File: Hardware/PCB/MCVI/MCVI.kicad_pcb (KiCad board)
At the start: 2 copper layers, 125.5 x 138 mm, 69 parts, among them IC1 TL074, IC2 TL074, J1 Synth_power_2x5, J10 AudioJack2, J11 AudioJack2, J12 AudioJack2, J13 AudioJack2, J14 AudioJack2, J15 AudioJack2, J16 AudioJack2, J2 10 pin header, J3 3 pin Molex header, J4 2 pin Molex header, J8 10 pin socket, J9 AudioJack2, U1 6N137

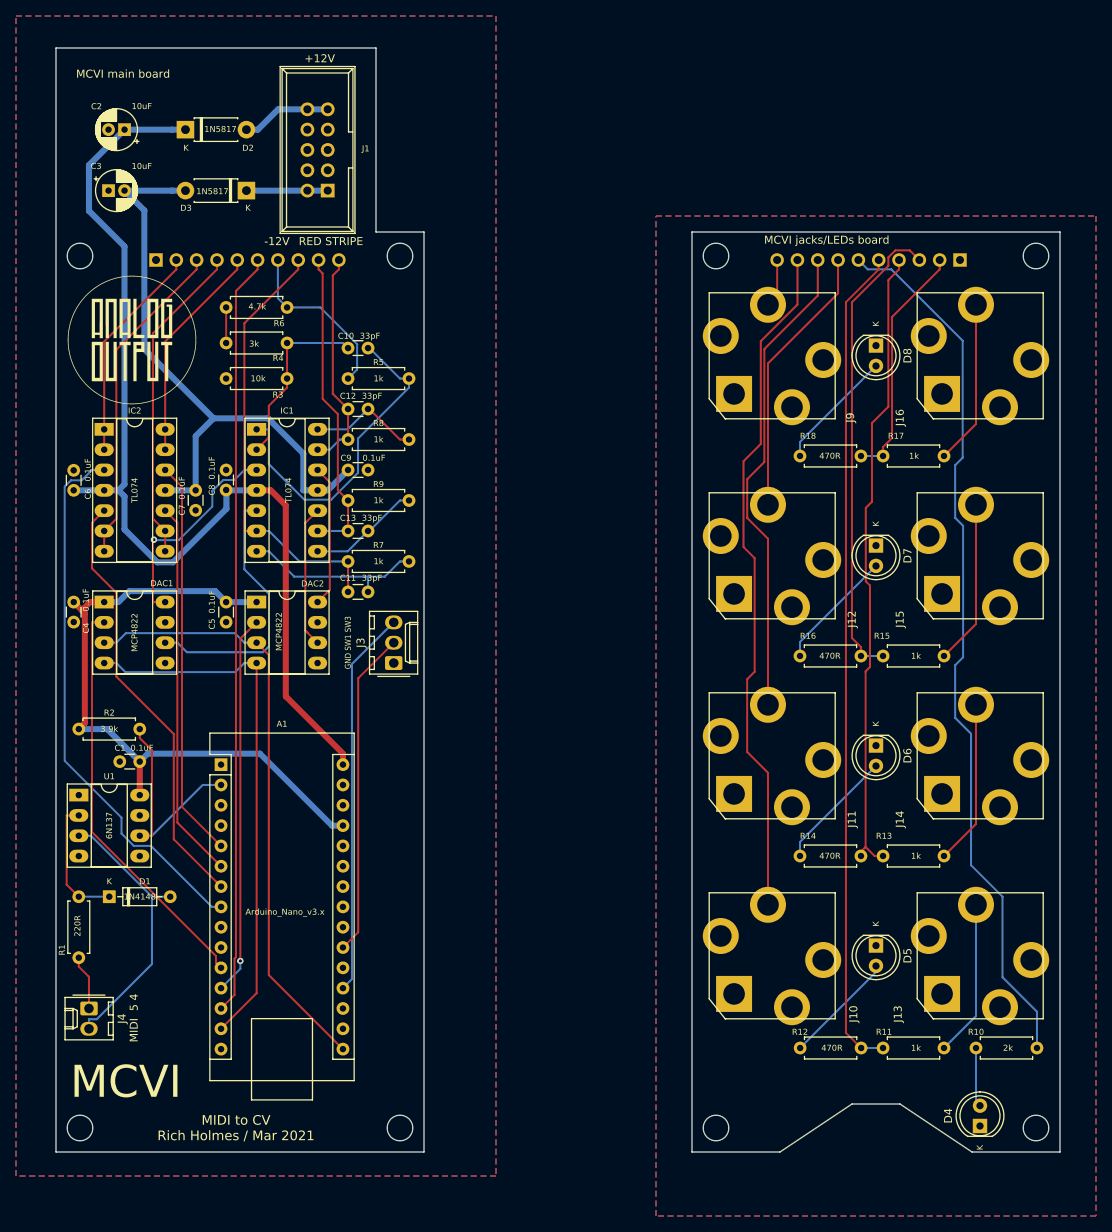
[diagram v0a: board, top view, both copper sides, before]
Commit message: Gerbers, docs updates
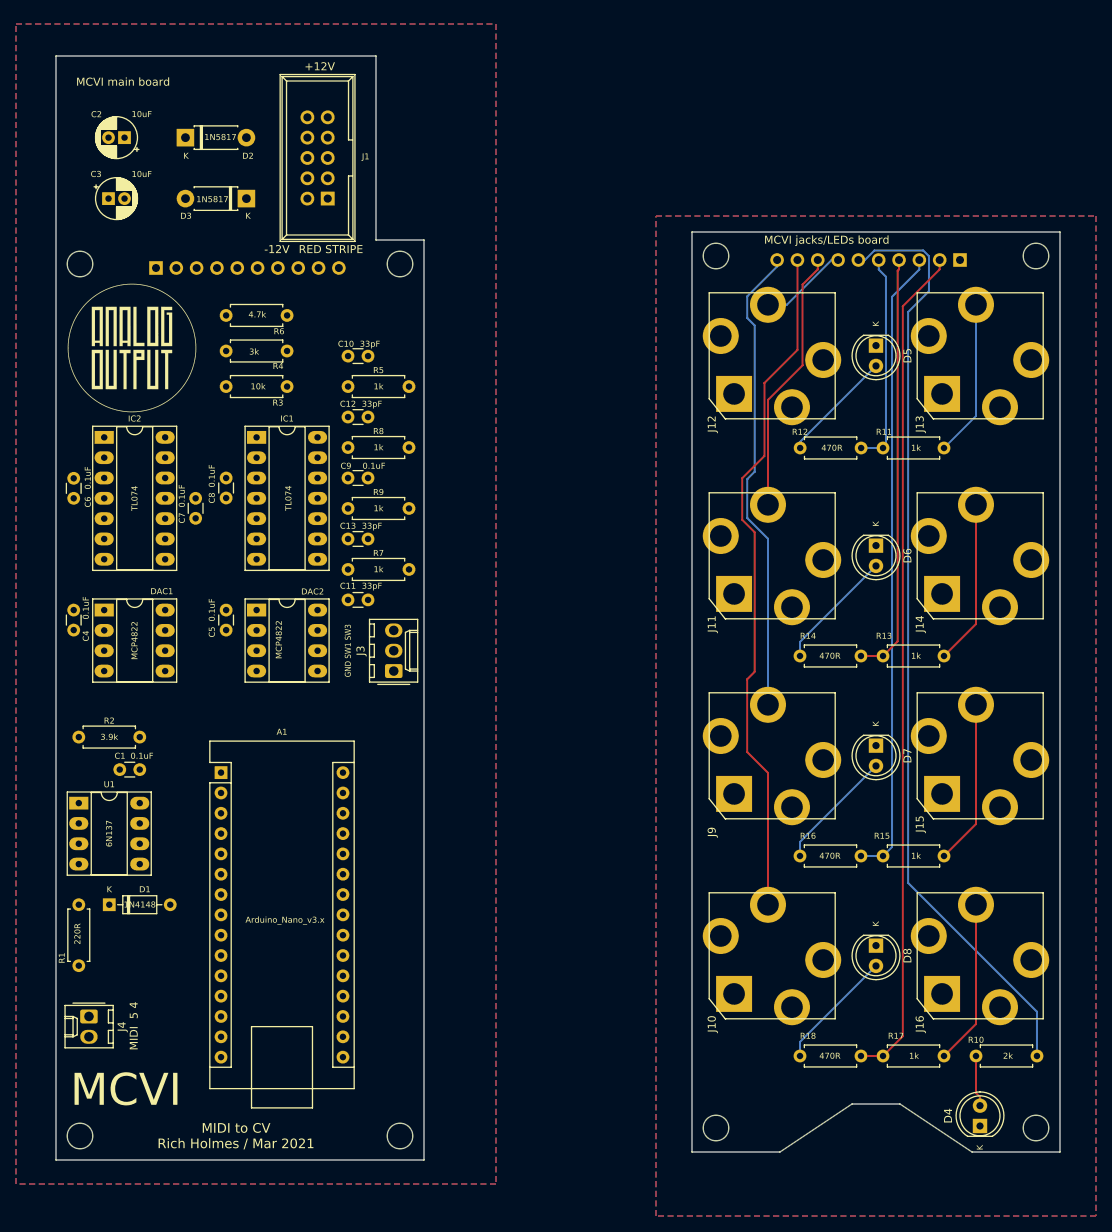
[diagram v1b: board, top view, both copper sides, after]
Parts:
- moved J13 75.0 mm to (155.0, 79.5)
- moved J16 75.0 mm to (155.0, 154.5)
- moved R11 75.0 mm to (150.5, 91.0)
- moved R12 75.0 mm to (132.5, 91.0)
- moved R17 75.0 mm to (150.5, 167.0)
- moved R18 75.0 mm to (132.5, 167.0)
- moved D5 75.0 mm to (142.0, 78.2)
- moved D8 75.0 mm to (142.0, 153.2)
- moved J9 50.0 mm to (129.0, 129.5)
- moved J11 25.0 mm to (129.0, 104.5)
- moved J12 25.0 mm to (129.0, 79.5)
- moved J14 25.0 mm to (155.0, 104.5)
- moved J15 25.0 mm to (155.0, 129.5)
- moved R13 25.0 mm to (150.5, 117.0)
- moved R14 25.0 mm to (132.5, 117.0)
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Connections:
- A1 pad 1: Net-(A1-Pad1) -> (no net)
- A1 pad 10: Net-(A1-Pad10) -> (no net)
- A1 pad 11: /DAC1_SEL -> (no net)
- A1 pad 12: /DAC2_SEL -> (no net)
- A1 pad 13: /MIDI_LED_A -> (no net)
- A1 pad 14: /SDI -> (no net)
- A1 pad 15: Net-(A1-Pad15) -> (no net)
- A1 pad 16: /SCK -> (no net)
- A1 pad 17: Net-(A1-Pad17) -> (no net)
- A1 pad 18: Net-(A1-Pad18) -> (no net)
- A1 pad 19: /SW3 -> (no net)
- A1 pad 2: /RX0 -> (no net)
- A1 pad 20: Net-(A1-Pad20) -> (no net)
- A1 pad 21: /SW1 -> (no net)
- A1 pad 22: Net-(A1-Pad22) -> (no net)
- A1 pad 23: Net-(A1-Pad23) -> (no net)
- A1 pad 24: Net-(A1-Pad24) -> (no net)
- A1 pad 25: Net-(A1-Pad25) -> (no net)
- A1 pad 26: Net-(A1-Pad26) -> (no net)
- A1 pad 27: +5V -> (no net)
- A1 pad 28: Net-(A1-Pad28) -> (no net)
- A1 pad 29: GND -> (no net)
- A1 pad 3: Net-(A1-Pad3) -> (no net)
- A1 pad 30: +12V -> (no net)
- A1 pad 4: GND -> (no net)
- A1 pad 5: /GATE_B -> (no net)
- A1 pad 6: /TRIGGER_B -> (no net)
- A1 pad 7: /CLOCK_1PQ_B -> (no net)
- A1 pad 8: /CLOCK_4PQ_B -> (no net)
- A1 pad 9: Net-(A1-Pad9) -> (no net)
- C1 pad 1: GND -> (no net)
- C1 pad 2: +5V -> (no net)
- C10 pad 1: Net-(C10-Pad1) -> (no net)
- C10 pad 2: Net-(C10-Pad2) -> (no net)
- C11 pad 1: Net-(C11-Pad1) -> (no net)
- C11 pad 2: /VELOCITY_A -> (no net)
- C12 pad 1: Net-(C12-Pad1) -> (no net)
- C12 pad 2: /PITCH_BEND_A -> (no net)
- C13 pad 1: Net-(C13-Pad1) -> (no net)
- C13 pad 2: /CONTROL_A -> (no net)
- C2 pad 1: +12V -> (no net)
- C2 pad 2: GND -> (no net)
- C3 pad 1: GND -> (no net)
- C3 pad 2: -12V -> (no net)
- C4 pad 1: +5V -> (no net)
- C4 pad 2: GND -> (no net)
- C5 pad 1: +5V -> (no net)
- C5 pad 2: GND -> (no net)
- C6 pad 1: +12V -> (no net)
- C6 pad 2: GND -> (no net)
- C7 pad 1: GND -> (no net)
- C7 pad 2: -12V -> (no net)
- C8 pad 1: +12V -> (no net)
- C8 pad 2: GND -> (no net)
- C9 pad 1: GND -> (no net)
- C9 pad 2: -12V -> (no net)
- D1 pad 1: Net-(D1-Pad1) -> (no net)
- D1 pad 2: /MIDIPIN5 -> (no net)
- D2 pad 1: +12V -> (no net)
- D2 pad 2: Net-(D2-Pad2) -> (no net)
- D3 pad 1: Net-(D3-Pad1) -> (no net)
- D3 pad 2: -12V -> (no net)
- DAC1 pad 1: +5V -> (no net)
- DAC1 pad 2: /DAC1_SEL -> (no net)
- DAC1 pad 3: /SCK -> (no net)
- DAC1 pad 4: /SDI -> (no net)
- DAC1 pad 5: GND -> (no net)
- DAC1 pad 6: /VELOCITY_B -> (no net)
- DAC1 pad 7: GND -> (no net)
- DAC1 pad 8: /NOTE_B -> (no net)
- DAC2 pad 1: +5V -> (no net)
- DAC2 pad 2: /DAC2_SEL -> (no net)
- DAC2 pad 3: /SCK -> (no net)
- DAC2 pad 4: /SDI -> (no net)
- DAC2 pad 5: GND -> (no net)
- DAC2 pad 6: /CONTROL_B -> (no net)
- DAC2 pad 7: GND -> (no net)
- DAC2 pad 8: /PITCH_BEND_B -> (no net)
- IC1 pad 1: Net-(C10-Pad1) -> (no net)
- IC1 pad 10: /CONTROL_B -> (no net)
- IC1 pad 11: -12V -> (no net)
- IC1 pad 12: /PITCH_BEND_B -> (no net)
- IC1 pad 13: /PITCH_BEND_A -> (no net)
- IC1 pad 14: Net-(C12-Pad1) -> (no net)
- IC1 pad 2: Net-(C10-Pad2) -> (no net)
- IC1 pad 3: /NOTE_B -> (no net)
- IC1 pad 4: +12V -> (no net)
- IC1 pad 5: /VELOCITY_B -> (no net)
- IC1 pad 6: /VELOCITY_A -> (no net)
- IC1 pad 7: Net-(C11-Pad1) -> (no net)
- IC1 pad 8: Net-(C13-Pad1) -> (no net)
- IC1 pad 9: /CONTROL_A -> (no net)
- IC2 pad 1: /CLOCK_4PQ_A -> (no net)
- IC2 pad 10: /TRIGGER_B -> (no net)
- IC2 pad 11: -12V -> (no net)
- IC2 pad 12: /GATE_B -> (no net)
- IC2 pad 13: /GATE_A -> (no net)
- IC2 pad 14: /GATE_A -> (no net)
- IC2 pad 2: /CLOCK_4PQ_A -> (no net)
- IC2 pad 3: /CLOCK_4PQ_B -> (no net)
- IC2 pad 4: +12V -> (no net)
- IC2 pad 5: /CLOCK_1PQ_B -> (no net)
- IC2 pad 6: /CLOCK_1PQ_A -> (no net)
- IC2 pad 7: /CLOCK_1PQ_A -> (no net)
- IC2 pad 8: /TRIGGER_A -> (no net)
- IC2 pad 9: /TRIGGER_A -> (no net)
- J1 pad 1: Net-(D3-Pad1) -> (no net)
- J1 pad 10: Net-(D2-Pad2) -> (no net)
- J1 pad 2: Net-(D3-Pad1) -> (no net)
- J1 pad 3: GND -> (no net)
- J1 pad 4: GND -> (no net)
- J1 pad 5: GND -> (no net)
- J1 pad 6: GND -> (no net)
- J1 pad 7: GND -> (no net)
- J1 pad 8: GND -> (no net)
- J1 pad 9: Net-(D2-Pad2) -> (no net)
- J2 pad 1: GND -> (no net)
- J2 pad 10: /PITCH_BEND_A -> (no net)
- J2 pad 2: /CLOCK_4PQ_A -> (no net)
- J2 pad 3: /CLOCK_1PQ_A -> (no net)
- J2 pad 4: /TRIGGER_A -> (no net)
- J2 pad 5: /GATE_A -> (no net)
- J2 pad 6: /MIDI_LED_A -> (no net)
- J2 pad 7: /NOTE_A -> (no net)
- J2 pad 8: /VELOCITY_A -> (no net)
- J2 pad 9: /CONTROL_A -> (no net)
- J3 pad 1: GND -> (no net)
- J3 pad 2: /SW1 -> (no net)
- J3 pad 3: /SW3 -> (no net)
- J4 pad 1: /MIDIPIN4 -> (no net)
- J4 pad 2: /MIDIPIN5 -> (no net)
- R1 pad 1: Net-(D1-Pad1) -> (no net)
- R1 pad 2: /MIDIPIN4 -> (no net)
- R2 pad 1: +5V -> (no net)
- R2 pad 2: /RX0 -> (no net)
- R3 pad 1: GND -> (no net)
- R3 pad 2: Net-(C10-Pad2) -> (no net)
- R4 pad 1: Net-(R4-Pad1) -> (no net)
- R4 pad 2: Net-(C10-Pad2) -> (no net)
- R5 pad 1: /NOTE_A -> (no net)
- R5 pad 2: Net-(C10-Pad1) -> (no net)
- R6 pad 1: /NOTE_A -> (no net)
- R6 pad 2: Net-(R4-Pad1) -> (no net)
- R7 pad 1: /VELOCITY_A -> (no net)
- R7 pad 2: Net-(C11-Pad1) -> (no net)
- R8 pad 1: /PITCH_BEND_A -> (no net)
- R8 pad 2: Net-(C12-Pad1) -> (no net)
- R9 pad 1: /CONTROL_A -> (no net)
- R9 pad 2: Net-(C13-Pad1) -> (no net)
- U1 pad 1: Net-(U1-Pad1) -> (no net)
- U1 pad 2: Net-(D1-Pad1) -> (no net)
- U1 pad 3: /MIDIPIN5 -> (no net)
- U1 pad 5: GND -> (no net)
- U1 pad 6: /RX0 -> (no net)
- U1 pad 7: Net-(U1-Pad7) -> (no net)
- U1 pad 8: +5V -> (no net)
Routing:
- net +12V: track 130.0 -> 0.00 mm
- net /MIDI_LED_A: track 95.5 -> 0.00 mm
- net +5V: track 83.2 -> 0.00 mm
- net -12V: track 78.7 -> 0.00 mm
- net /Panel components/GATE_C: track 103.7 -> 26.8 mm
- net /SCK: track 75.3 -> 0.00 mm
- net /Panel components/CLOCK_4PQ_C: track 30.2 -> 105.2 mm
- net /CLOCK_4PQ_B: track 68.3 -> 0.00 mm
- net /SDI: track 67.6 -> 0.00 mm
- net /VELOCITY_A: track 55.0 -> 0.00 mm
- net /CLOCK_1PQ_B: track 54.3 -> 0.00 mm
- net /Panel components/PITCH_BEND: track 6.07 -> 59.0 mm
- net /DAC1_SEL: track 51.4 -> 0.00 mm
- net /GATE_B: track 49.9 -> 0.00 mm
- net /SW3: track 48.4 -> 0.00 mm
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- added copper zone on B.Cu, net (none)
- added copper zone on F.Cu, net (none)
- removed copper zone on B.Cu, net GND
- removed copper zone on F.Cu, net GND
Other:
- outline, holes or cut-outs redrawn
